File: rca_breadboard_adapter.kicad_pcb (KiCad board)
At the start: 2 copper layers, 22.9 x 22.9 mm, 4 parts, among them J1 Conn_Coaxial, J2 Conn_Coaxial, J3 Conn_02x03_Odd_Even, J4 Conn_02x03_Odd_Even

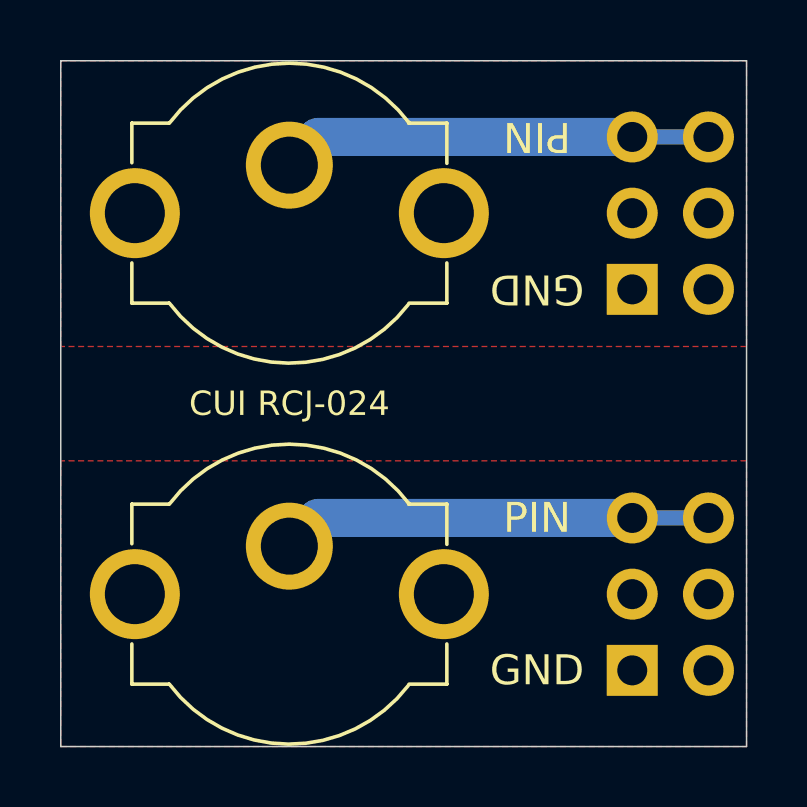
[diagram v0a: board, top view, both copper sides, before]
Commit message: Update project to kicad 6+
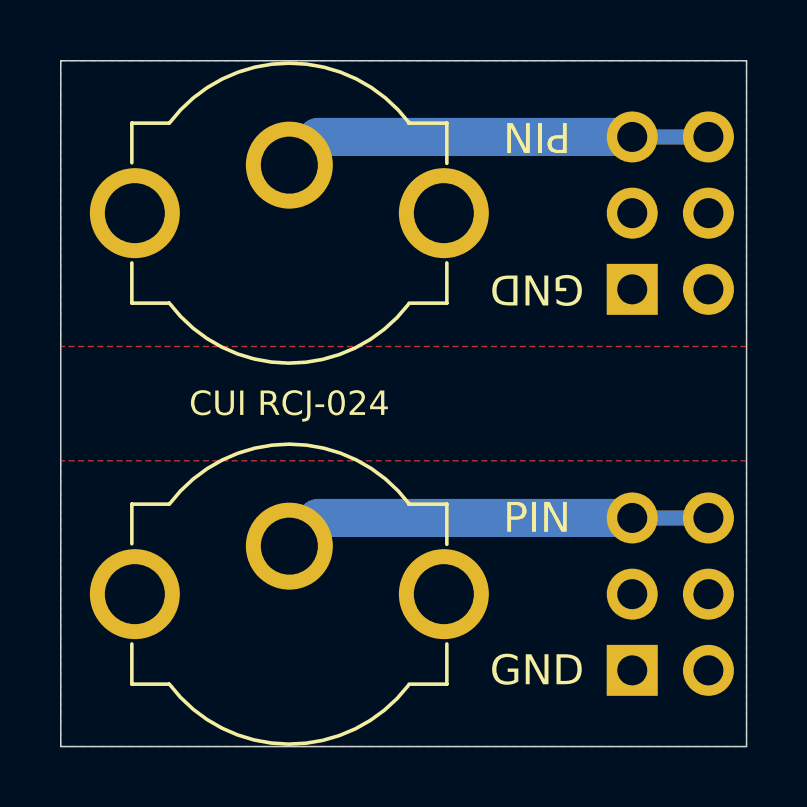
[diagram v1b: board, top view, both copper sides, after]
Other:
- net class Default removed
